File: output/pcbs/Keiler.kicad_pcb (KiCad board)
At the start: 2 copper layers, 133.9 x 103.2 mm, 44 parts

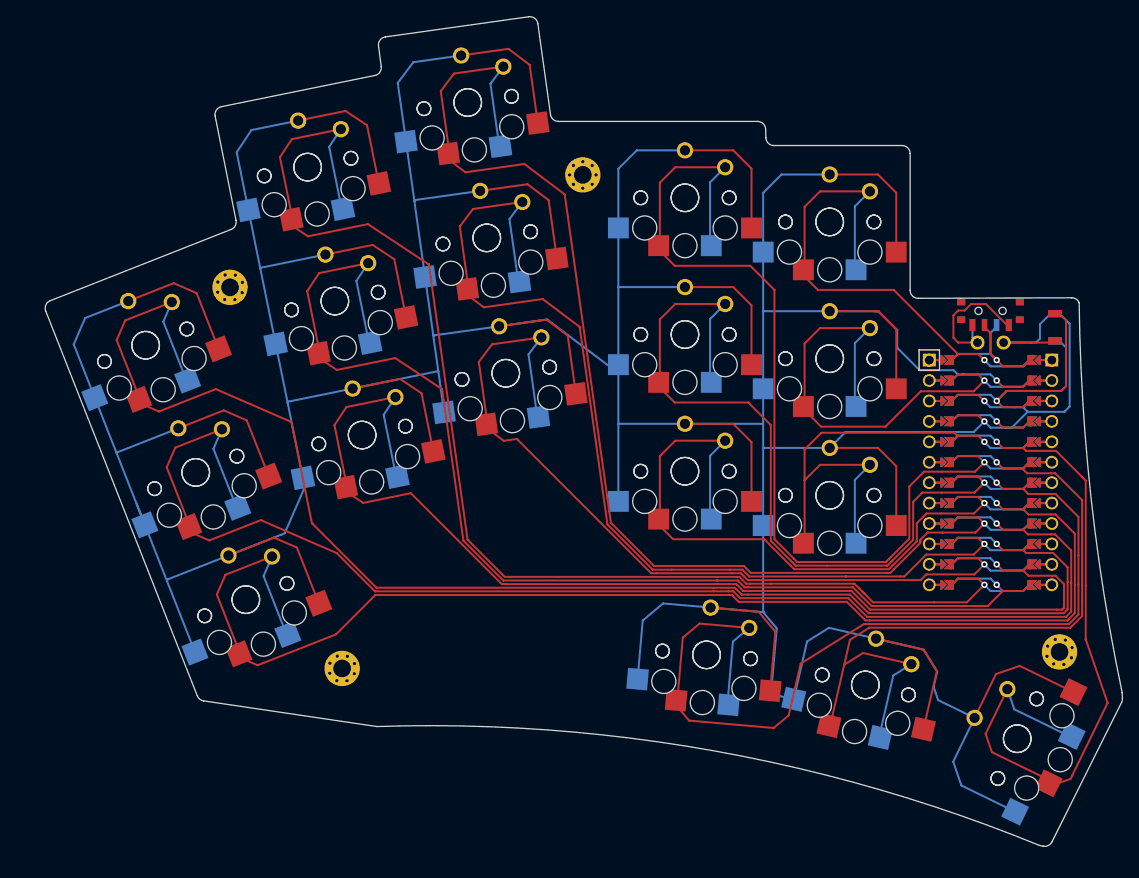
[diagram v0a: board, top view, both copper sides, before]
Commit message: Nicer routing
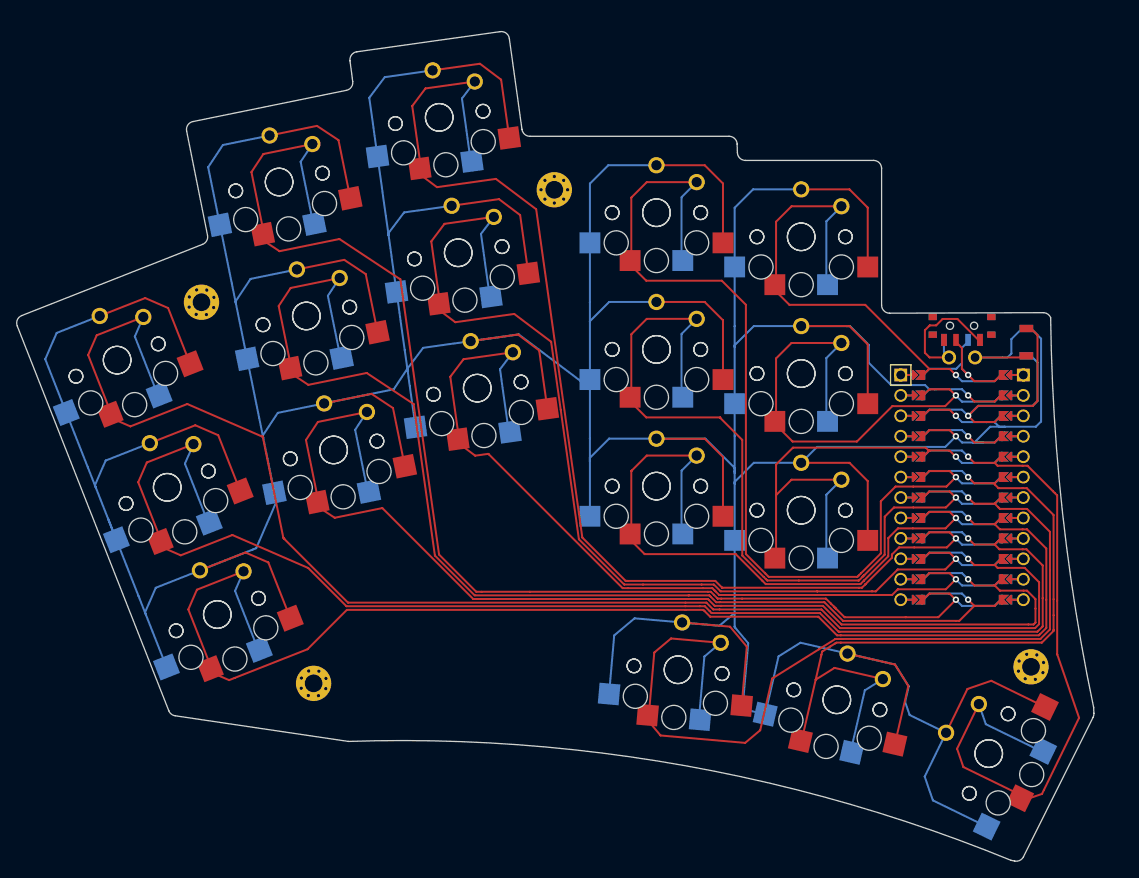
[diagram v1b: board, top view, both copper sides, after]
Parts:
- moved S16 4.00 mm to (182.4, 169.6)
- moved S34 4.00 mm to (182.4, 169.6)
- moved S15 4.00 mm to (197.7, 115.8)
- moved S33 4.00 mm to (197.7, 115.8)
- moved _7 4.00 mm to (167.0, 109.9)
- moved S27 4.00 mm to (152.7, 100.9)
- moved S9 4.00 mm to (152.7, 100.9)
- moved MCU1 4.00 mm to (217.7, 146.9)
- moved S22 4.00 mm to (139.6, 142.3)
- moved S4 4.00 mm to (139.6, 142.3)
- moved S21 4.00 mm to (112.7, 131.1)
- moved S3 4.00 mm to (112.7, 131.1)
- moved S17 4.00 mm to (202.2, 173.3)
- moved S35 4.00 mm to (202.2, 173.3)
- moved S1 4.00 mm to (125.1, 162.7)
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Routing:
- net GND: track 902.5 -> 919.7 mm
- net P19: track 118.0 -> 118.7 mm
